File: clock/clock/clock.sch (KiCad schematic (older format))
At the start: 44 parts, among them J1 AVR-ISP-6, J10 Conn_01x07_Male, J11 CV_IN, J12 CLOCK_OUT, J13 SUBDIV_OUT, J2 EURORACK_CONN_10, J3 Conn_01x05_Female, J4 Conn_01x05_Male, J5 Conn_01x05_Female, J6 Conn_01x05_Male, J7 Conn_01x05_Female, J8 Conn_01x05_Male, J9 Conn_01x07_Female, SW1 SW_Push, SW2 SW_Push, SW3 Rotary_Encoder_Switch, U1 ATmega328P-PU, U2 L7805, U3 SM460281N, U4 SM460281N, U5 SM460281N, Y1 16MHz

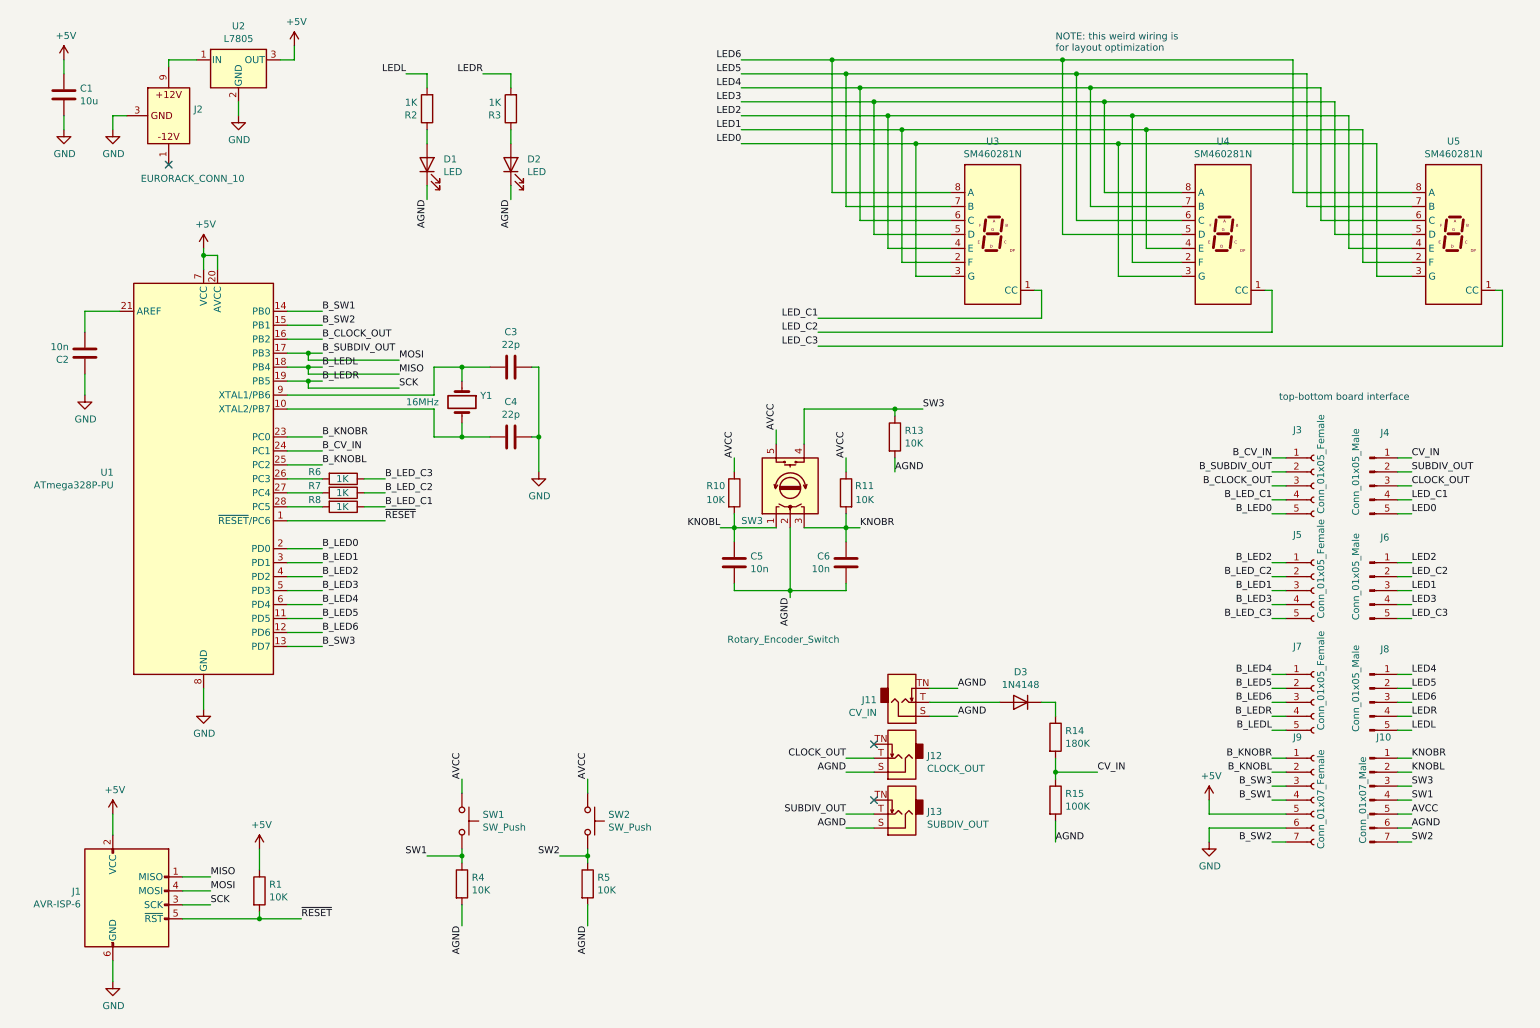
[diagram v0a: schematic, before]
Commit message: beautify schematic
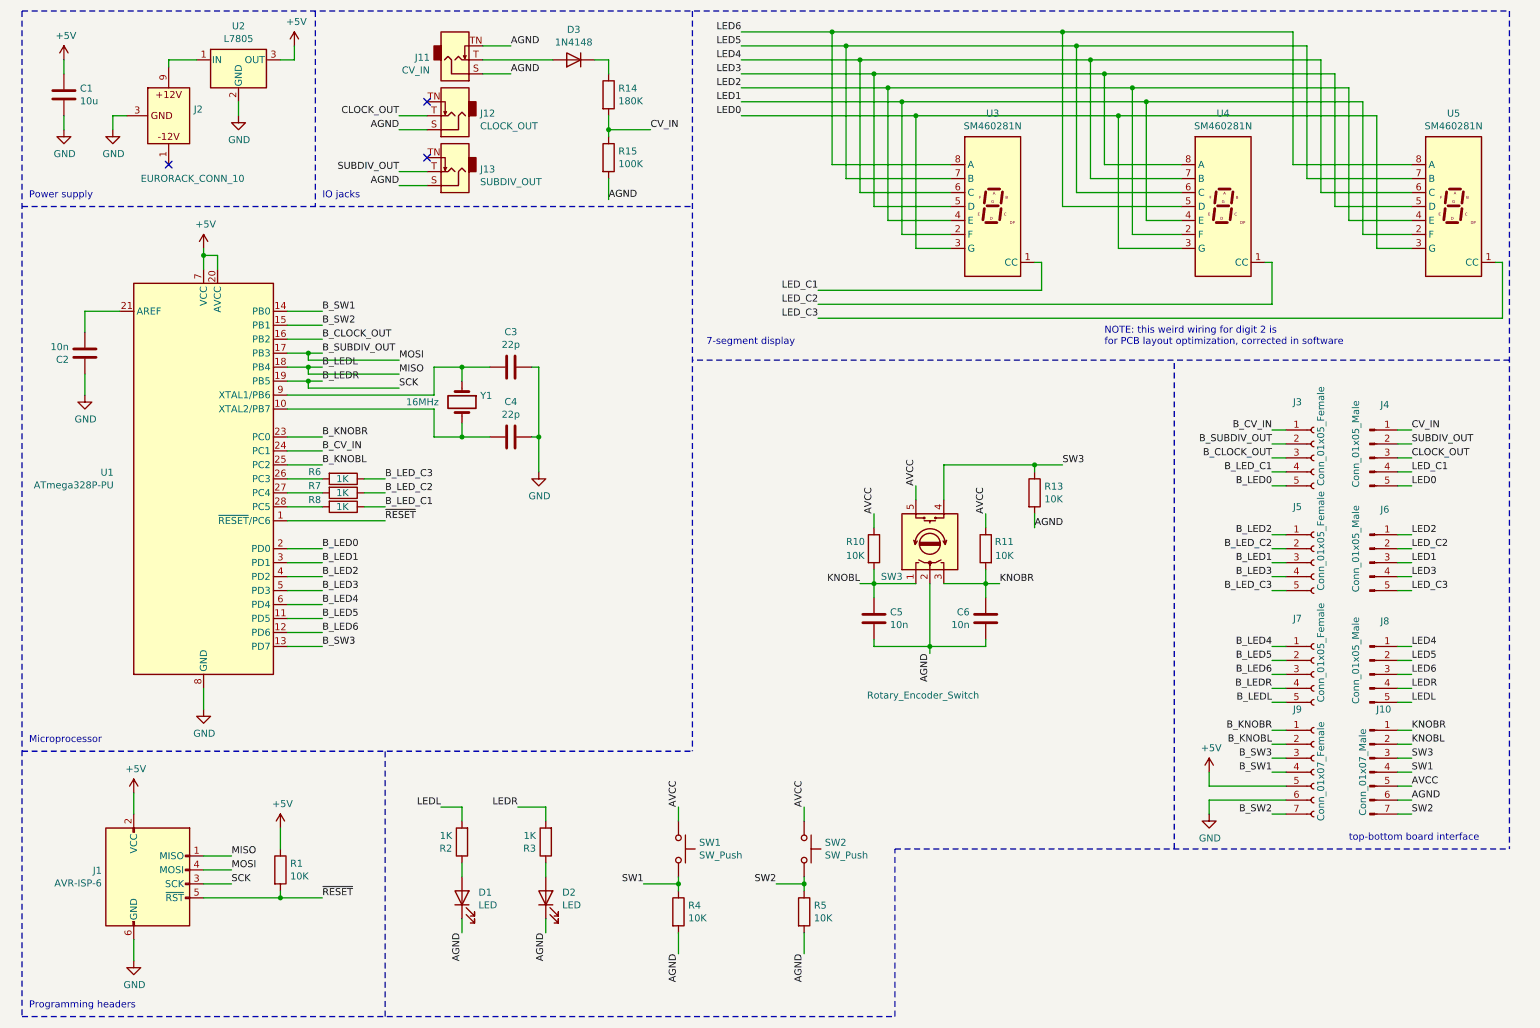
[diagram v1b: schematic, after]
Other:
- note added: "7-segment display"
- note added: "IO jacks"
- note added: "Microprocessor"
- note added: "NOTE: this weird wiring for digit 2 is\nfor PCB layout optimization, corrected in software"
- note added: "Power supply"
- note added: "Programming headers"
- note removed: "NOTE: this weird wiring is\nfor layout optimization"
- moved on the sheet: C5, C6, D1, D2, D3, J1, J10, J11, J12, J13, J3, J4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
